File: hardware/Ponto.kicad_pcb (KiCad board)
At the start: 2 copper layers, 47 x 30.5 mm, 8 parts, among them P1 RFID-RC522-MODULE, P2 CONN_01X04, U1 ESP-07v2, U2 LM1117-3.3

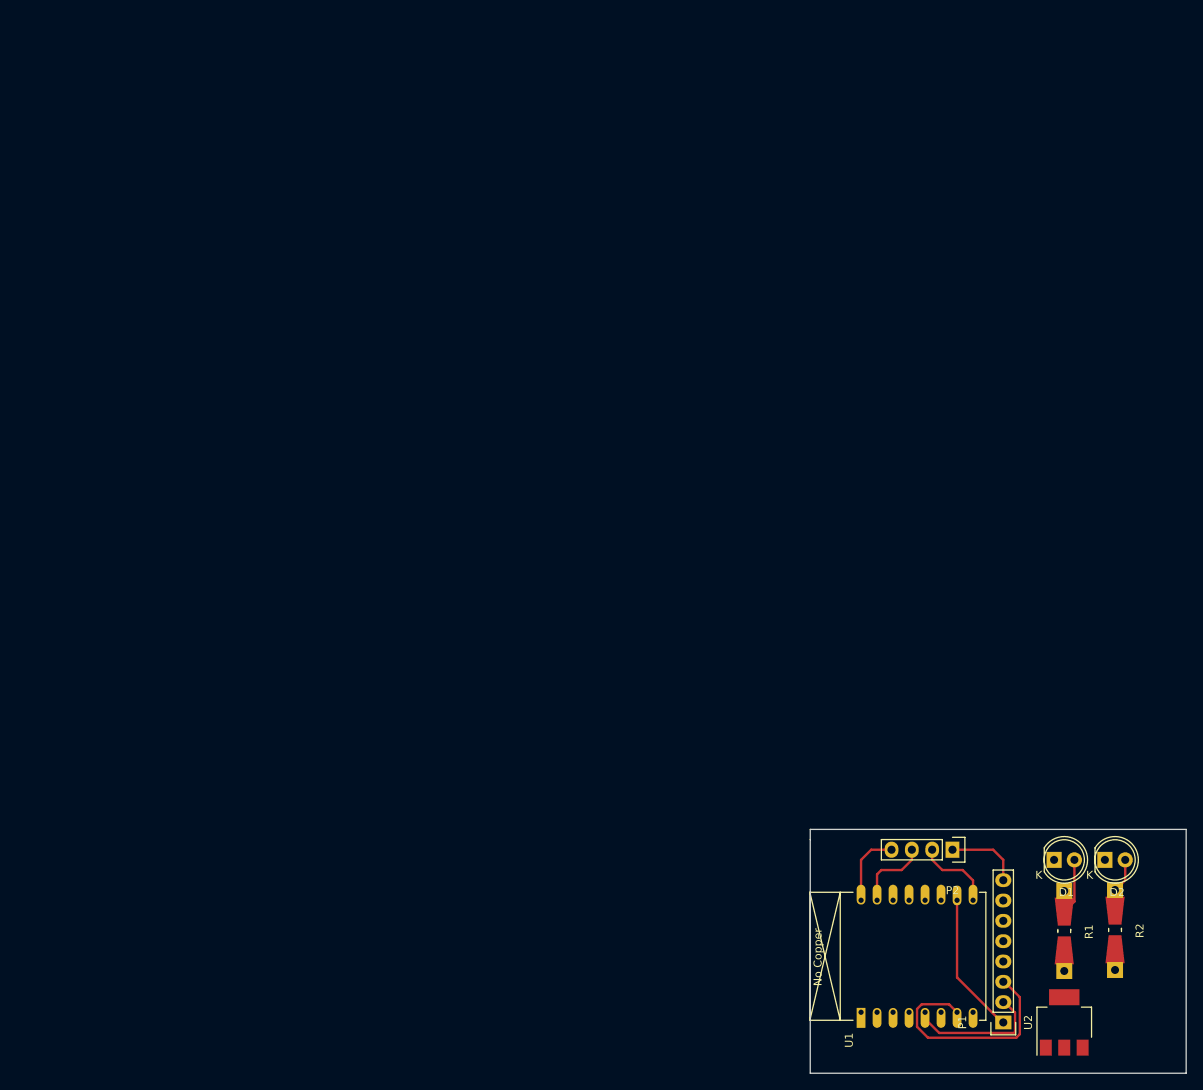
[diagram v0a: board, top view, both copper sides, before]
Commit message: Começando PCB
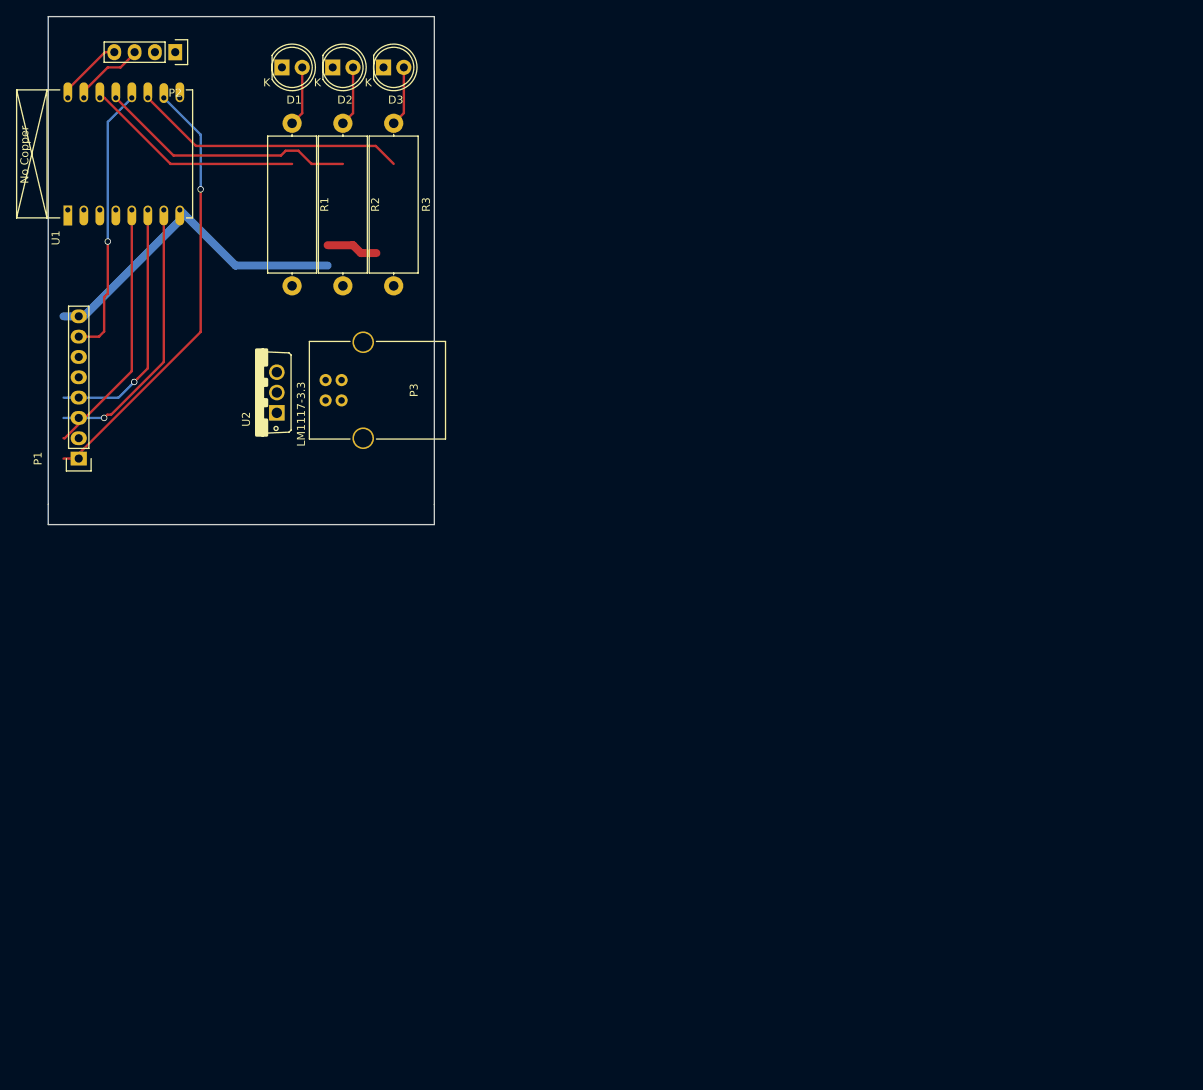
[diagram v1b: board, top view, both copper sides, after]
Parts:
- added D3: LED, LEDs:LED-5MM, F.Cu at (108.0, 31.8)
- added P3: USB_B, Connectors:USB_B, F.Cu at (100.7, 70.8)
- added R3: 4K7, Resistors_THT:R_Axial_DIN0617_L17.0mm_D6.0mm_P20.32mm_Horizontal, F.Cu at (109.2, 38.7)
- R1, R2: footprint Resistors_Universal:Resistor_SMD+THTuniversal_0805to1206_RM10_HandSoldering -> Resistors_THT:R_Axial_DIN0617_L17.0mm_D6.0mm_P20.32mm_Horizontal
- U2: footprint TO_SOT_Packages_SMD:SOT-223 -> Common-Parts-Library:TO-220-3
- moved U1 141.0 mm to (68.5, 49.6)
- moved R1 139.7 mm to (96.5, 38.7)
- moved R2 139.6 mm to (102.9, 38.7)
- moved P2 139.2 mm to (81.9, 29.8)
- moved D1 138.3 mm to (95.2, 31.8)
- moved D2 138.3 mm to (101.6, 31.8)
- moved P1 135.4 mm to (69.8, 80.6)
- moved U2 126.0 mm to (94.6, 72.4)
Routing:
- net SDA: track 17.8 -> 54.9 mm, vias 0 -> 1
- net Net-(R3-Pad2): track 0.00 -> 34.2 mm
- net RST: track 0.00 -> 34.1 mm, vias 0 -> 1
- net VCC: track 9.42 -> 42.2 mm
- net Net-(R2-Pad2): track 0.00 -> 32.3 mm
- net MISO: track 0.00 -> 31.9 mm, vias 0 -> 1
- net Net-(R1-Pad2): track 0.00 -> 27.5 mm
- net SCK: track 17.3 -> 32.2 mm
- net GND: track 9.92 -> 0.00 mm
- net Net-(D3-Pad2): track 0.00 -> 7.51 mm
- net Net-(P3-Pad1): track 0.00 -> 6.50 mm
- net MOSI: track 29.0 -> 34.4 mm, vias 0 -> 1
- net Net-(D2-Pad2): track 4.32 -> 7.51 mm
- net TX: track 9.39 -> 8.80 mm
- net Net-(D1-Pad2): track 7.00 -> 7.51 mm
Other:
- board size 47 x 30.5 mm -> 48.3 x 63.5 mm
